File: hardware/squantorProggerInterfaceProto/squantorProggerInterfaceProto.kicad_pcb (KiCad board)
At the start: 2 copper layers, 15.9 x 20.9 mm, 24 parts, among them J1 JTAG_interface_proto_input, J2 JTAG_interface_proto_output, U1 74X1T45, U2 74X1T45, U3 74X1T45, U4 74X1T45, U5 74X1G125

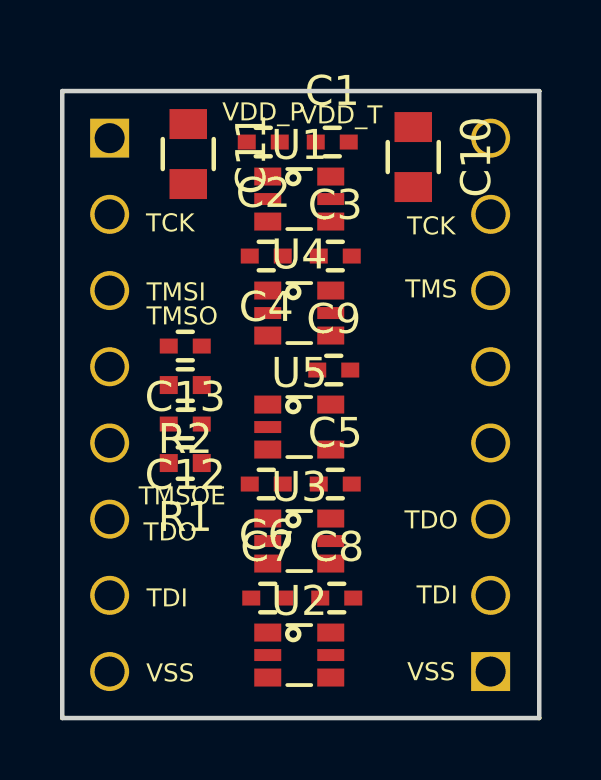
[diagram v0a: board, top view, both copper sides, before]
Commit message: routing completed, no DRC errors
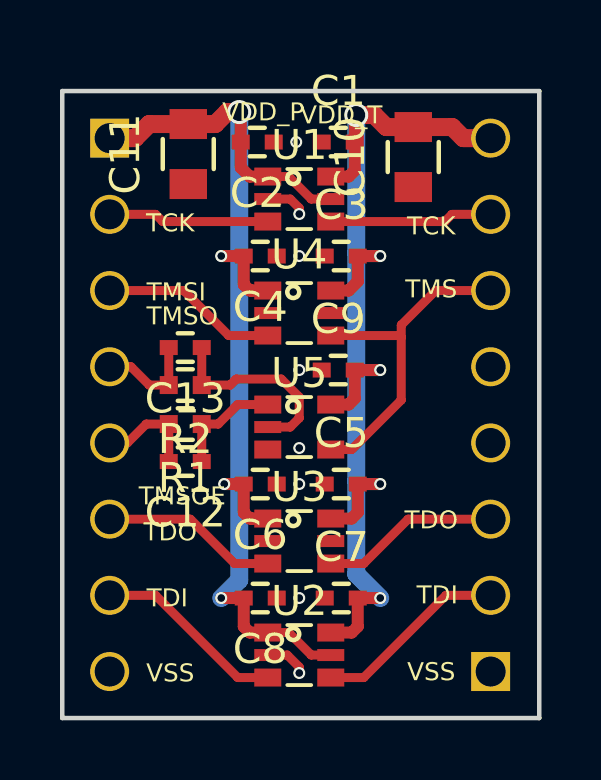
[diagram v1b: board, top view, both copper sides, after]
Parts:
- moved C8 2.55 mm to (149.8, 92.8), turned to 180 degrees
- moved C7 2.45 mm to (152.5, 92.8)
- moved R1 1.30 mm to (147.3, 87.0)
- moved C12 1.25 mm to (147.3, 88.2)
- moved C1 0.20 mm to (152.4, 77.6)
- moved C2 0.20 mm to (149.7, 77.6)
- moved C3 0.20 mm to (152.5, 81.4)
- moved C4 0.20 mm to (149.8, 81.4)
- moved C5 0.20 mm to (152.5, 89.0)
- moved C6 0.20 mm to (149.8, 89.0)
- moved C9 0.15 mm to (152.4, 85.2)
- turned C10 to 90 degrees
- turned C11 to 90 degrees
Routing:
- net /VDD_PROG: track 0.00 -> 37.6 mm, vias 0 -> 4
- net /VDD_TARGET: track 0.00 -> 37.2 mm, vias 0 -> 5
- net /TMS_TARGET: track 0.00 -> 11.4 mm
- net Net-(C13-Pad1): track 0.00 -> 6.73 mm
- net /TDI_TARGET: track 0.00 -> 6.46 mm
- net /TDI_PROG: track 0.00 -> 6.40 mm
- net /TDO_TARGET: track 0.00 -> 5.94 mm
- net /TMSI_PROG: track 0.00 -> 5.89 mm
- net /TDO_PROG: track 0.00 -> 5.88 mm
- net /TCK_TARGET: track 0.00 -> 5.43 mm
- net /TCK_PROG: track 0.00 -> 5.37 mm
- net Net-(C12-Pad1): track 0.00 -> 3.74 mm
- net /TMSO_PROG: track 0.00 -> 3.49 mm
- net /TMSOE_PROG: track 0.00 -> 3.45 mm
- net /VSS: track 0.00 -> 2.79 mm, vias 0 -> 8
- added copper zone on B.Cu, net /VSS
- added copper zone on F.Cu, net /VSS
